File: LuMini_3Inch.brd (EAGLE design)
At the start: 76.2 x 76.2 mm, 37 parts, among them J1 SOLDER_PAD_2, J2 SOLDER_PAD_2, J3 SOLDER_PAD_2

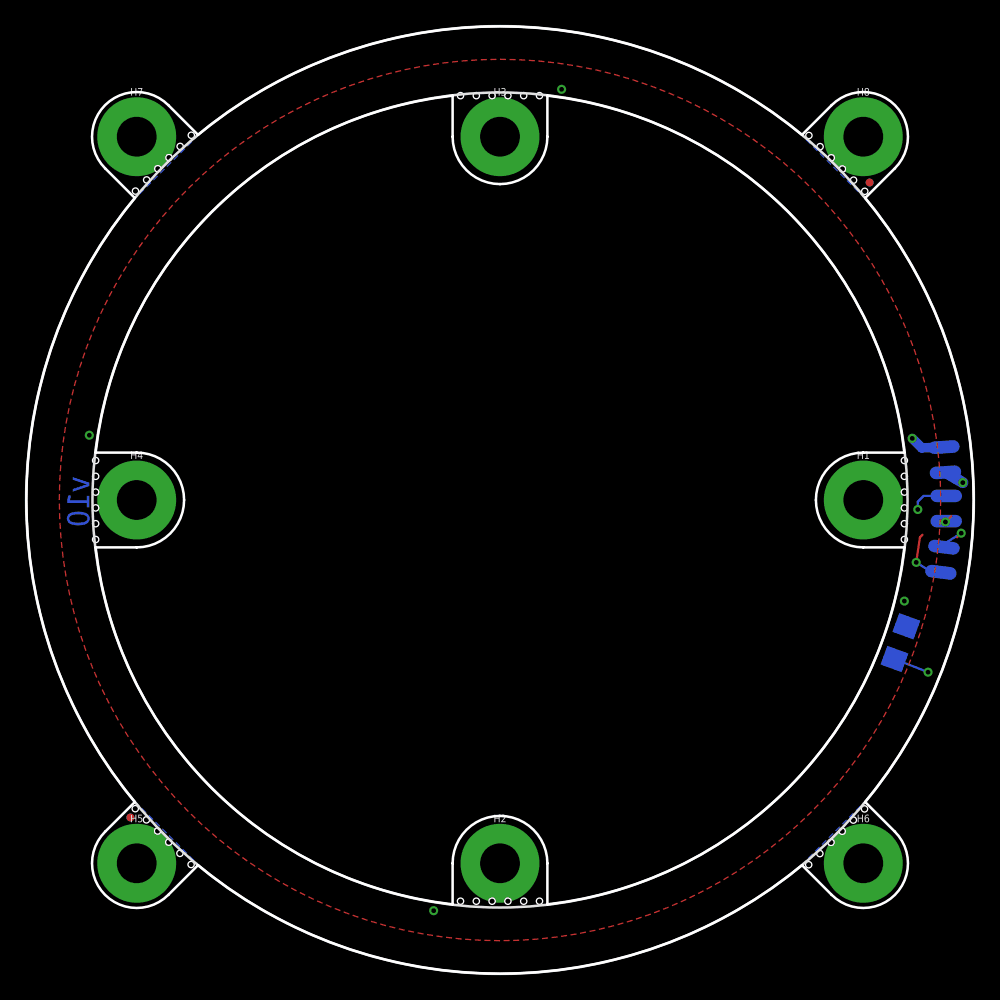
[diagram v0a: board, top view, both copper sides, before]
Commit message: about to repin IVL
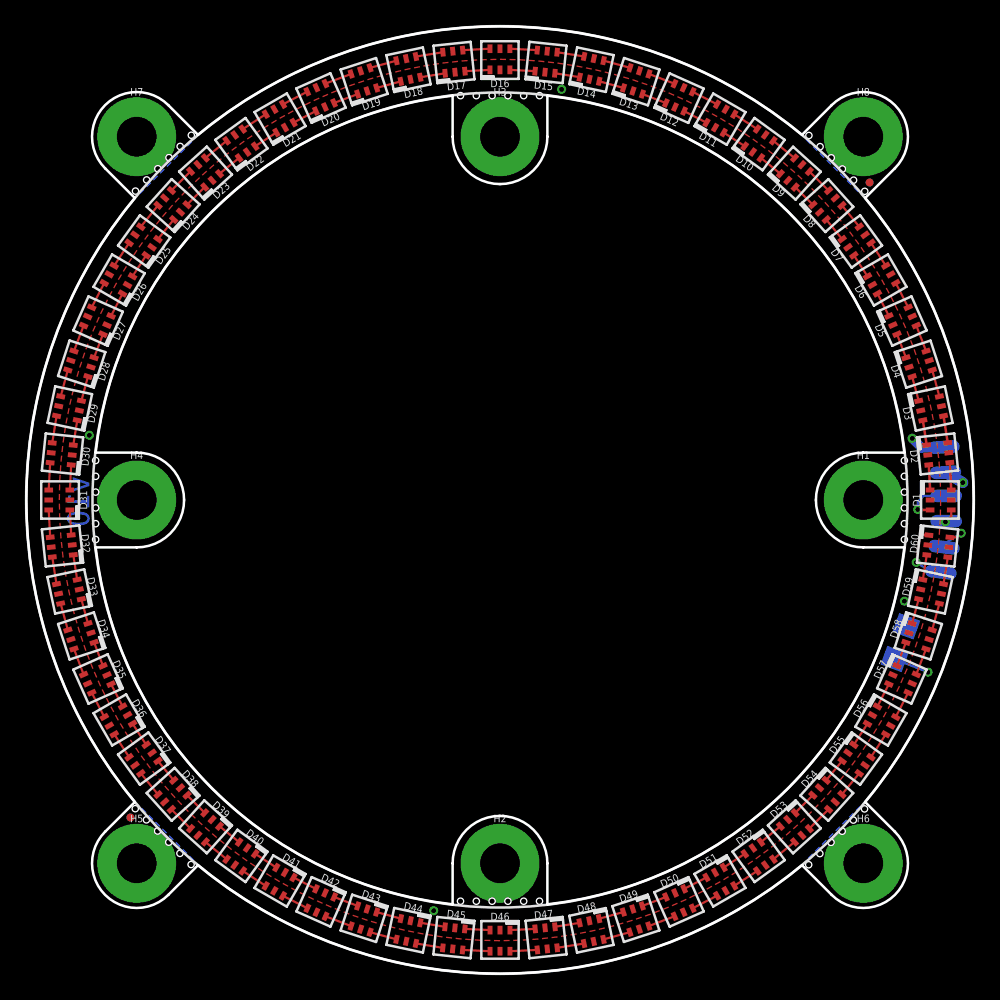
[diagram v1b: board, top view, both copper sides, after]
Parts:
- added D1, D10, D11, D12, D13, D14, D15, D16, D17, D18, D19, D2, D20, D21, D22, D23, D24, D25, D26, D27, D28, D29, D3, D30, D31, D32, D33, D34, D35, D36, D37, D38, D39, D4, D40, D41, D42, D43, D44, D45, D46, D47, D48, D49, D5, D50, D51, D52, D53, D54, D55, D56, D57, D58, D59, D6, D60, D7, D8, D9: APA102-2020, SparkFun-LED:APA102-2020
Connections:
- new net N$1: D4.CKO, D5.CKI
- new net N$10: D4.SDO, D5.SDI
- new net N$100: D50.CKO, D51.CKI
- new net N$101: D50.SDO, D51.SDI
- new net N$102: D51.CKO, D52.CKI
- new net N$103: D51.SDO, D52.SDI
- new net N$104: D52.CKO, D53.CKI
- new net N$105: D52.SDO, D53.SDI
- new net N$106: D53.CKO, D54.CKI
- new net N$107: D53.SDO, D54.SDI
- new net N$108: D54.CKO, D55.CKI
- new net N$109: D54.SDO, D55.SDI
- new net N$11: D5.CKO, D6.CKI
- new net N$110: D55.CKO, D56.CKI
- new net N$111: D55.SDO, D56.SDI
- new net N$112: D57.CKO, D58.CKI
- new net N$113: D57.SDO, D58.SDI
- new net N$114: D58.SDO, D59.SDI
- new net N$115: D59.CKO, D60.CKI
- new net N$116: D59.SDO, D60.SDI
- new net N$117: D58.CKO, D59.CKI
- new net N$118: D48.CKO, D49.CKI
- new net N$119: D48.SDO, D49.SDI
- new net N$12: D5.SDO, D6.SDI
- new net N$120: D56.SDO, D57.SDI
- new net N$121: D56.CKO, D57.CKI
- new net N$124: D20.CKO, D21.CKI
- new net N$13: D6.CKO, D7.CKI
- new net N$14: D6.SDO, D7.SDI
- new net N$15: D7.CKO, D8.CKI
- new net N$16: D7.SDO, D8.SDI
- new net N$17: D16.SDO, D17.SDI
- new net N$18: D20.SDO, D21.SDI
- new net N$19: D10.CKI, D9.CKO
- new net N$20: D10.SDI, D9.SDO
- new net N$21: D10.CKO, D11.CKI
- new net N$22: D10.SDO, D11.SDI
- new net N$23: D11.CKO, D12.CKI
- new net N$24: D11.SDO, D12.SDI
- new net N$25: D12.CKO, D13.CKI
- new net N$26: D12.SDO, D13.SDI
- new net N$27: D13.CKO, D14.CKI
- new net N$28: D13.SDO, D14.SDI
- new net N$29: D14.CKO, D15.CKI
- new net N$30: D14.SDO, D15.SDI
- new net N$31: D45.CKO, D46.CKI
- new net N$32: D30.CKO, D31.CKI
- new net N$33: D8.CKO, D9.CKI
- new net N$34: D8.SDO, D9.SDI
- new net N$35: D17.CKO, D18.CKI
- new net N$36: D17.SDO, D18.SDI
- new net N$37: D18.CKO, D19.CKI
- new net N$38: D18.SDO, D19.SDI
- new net N$39: D19.CKO, D20.CKI
- new net N$4: D1.CKO, D2.CKI
- new net N$40: D19.SDO, D20.SDI
- new net N$41: D30.SDO, D31.SDI
- new net N$42: D15.CKO, D16.CKI
- new net N$43: D16.CKO, D17.CKI
- new net N$44: D21.CKO, D22.CKI
- new net N$45: D21.SDO, D22.SDI
- new net N$46: D22.CKO, D23.CKI
- new net N$47: D22.SDO, D23.SDI
- new net N$48: D23.CKO, D24.CKI
- new net N$49: D23.SDO, D24.SDI
- new net N$5: D1.SDO, D2.SDI
- new net N$50: D24.CKO, D25.CKI
- new net N$51: D24.SDO, D25.SDI
- new net N$52: D25.CKO, D26.CKI
- new net N$53: D25.SDO, D26.SDI
- new net N$54: D26.CKO, D27.CKI
- new net N$55: D26.SDO, D27.SDI
- new net N$56: D27.CKO, D28.CKI
- new net N$57: D27.SDO, D28.SDI
- new net N$58: D29.CKO, D30.CKI
- new net N$59: D29.SDO, D30.SDI
- new net N$6: D2.CKO, D3.CKI
- new net N$60: D15.SDO, D16.SDI
- new net N$61: D45.SDO, D46.SDI
- new net N$62: D31.CKO, D32.CKI
- new net N$63: D31.SDO, D32.SDI
- new net N$64: D32.CKO, D33.CKI
- new net N$65: D32.SDO, D33.SDI
- new net N$66: D33.CKO, D34.CKI
- new net N$67: D33.SDO, D34.SDI
- new net N$68: D34.CKO, D35.CKI
- new net N$69: D34.SDO, D35.SDI
- new net N$7: D2.SDO, D3.SDI
- new net N$70: D35.CKO, D36.CKI
- new net N$71: D35.SDO, D36.SDI
- new net N$72: D37.CKO, D38.CKI
- new net N$73: D37.SDO, D38.SDI
- new net N$74: D38.SDO, D39.SDI
- new net N$75: D39.CKO, D40.CKI
- new net N$76: D39.SDO, D40.SDI
- new net N$77: D38.CKO, D39.CKI
- new net N$78: D28.CKO, D29.CKI
- new net N$79: D28.SDO, D29.SDI
- new net N$8: D3.CKO, D4.CKI
- new net N$80: D36.SDO, D37.SDI
- new net N$81: D36.CKO, D37.CKI
- new net N$82: D40.CKO, D41.CKI
- new net N$83: D40.SDO, D41.SDI
- new net N$84: D41.CKO, D42.CKI
- new net N$85: D41.SDO, D42.SDI
- new net N$86: D42.CKO, D43.CKI
- new net N$87: D42.SDO, D43.SDI
- new net N$88: D43.CKO, D44.CKI
- new net N$89: D43.SDO, D44.SDI
- new net N$9: D3.SDO, D4.SDI
- new net N$90: D44.CKO, D45.CKI
- new net N$91: D44.SDO, D45.SDI
- new net N$94: D46.CKO, D47.CKI
- new net N$95: D46.SDO, D47.SDI
- new net N$96: D47.CKO, D48.CKI
- new net N$97: D47.SDO, D48.SDI
- new net N$98: D49.CKO, D50.CKI
- new net N$99: D49.SDO, D50.SDI
- net 5V: now also D1.VDD, D10.VDD, D11.VDD, D12.VDD, D13.VDD, D14.VDD, D15.VDD, D16.VDD, D17.VDD, D18.VDD, D19.VDD, D2.VDD, D20.VDD, D21.VDD, D22.VDD, D23.VDD, D24.VDD, D25.VDD, D26.VDD, D27.VDD, D28.VDD, D29.VDD, D3.VDD, D30.VDD, D31.VDD, D32.VDD, D33.VDD, D34.VDD, D35.VDD, D36.VDD, D37.VDD, D38.VDD, D39.VDD, D4.VDD, D40.VDD, D41.VDD, D42.VDD, D43.VDD, D44.VDD, D45.VDD, D46.VDD, D47.VDD, D48.VDD, D49.VDD, D5.VDD, D50.VDD, D51.VDD, D52.VDD, D53.VDD, D54.VDD, D55.VDD, D56.VDD, D57.VDD, D58.VDD, D59.VDD, D6.VDD, D60.VDD, D7.VDD, D8.VDD, D9.VDD
- net CI: now also D1.CKI
- net CO: now also D60.CKO
- net DI: now also D1.SDI
- net DO: now also D60.SDO
- net GND: now also D1.GND, D10.GND, D11.GND, D12.GND, D13.GND, D14.GND, D15.GND, D16.GND, D17.GND, D18.GND, D19.GND, D2.GND, D20.GND, D21.GND, D22.GND, D23.GND, D24.GND, D25.GND, D26.GND, D27.GND, D28.GND, D29.GND, D3.GND, D30.GND, D31.GND, D32.GND, D33.GND, D34.GND, D35.GND, D36.GND, D37.GND, D38.GND, D39.GND, D4.GND, D40.GND, D41.GND, D42.GND, D43.GND, D44.GND, D45.GND, D46.GND, D47.GND, D48.GND, D49.GND, D5.GND, D50.GND, D51.GND, D52.GND, D53.GND, D54.GND, D55.GND, D56.GND, D57.GND, D58.GND, D59.GND, D6.GND, D60.GND, D7.GND, D8.GND, D9.GND
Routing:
- net N$98: track 0.00 -> 2.21 mm
- net N$15: track 0.00 -> 2.21 mm
- net N$75: track 0.00 -> 2.21 mm
- net N$31: track 0.00 -> 2.21 mm
- net N$50: track 0.00 -> 2.21 mm
- net N$4: track 0.00 -> 2.21 mm
- net N$42: track 0.00 -> 2.21 mm
- net N$94: track 0.00 -> 2.21 mm
- net N$39: track 0.00 -> 2.21 mm
- net N$1: track 0.00 -> 2.21 mm
- net N$44: track 0.00 -> 2.21 mm
- net N$117: track 0.00 -> 2.21 mm
- net N$54: track 0.00 -> 2.21 mm
- net N$19: track 0.00 -> 2.21 mm
- net N$108: track 0.00 -> 2.21 mm
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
